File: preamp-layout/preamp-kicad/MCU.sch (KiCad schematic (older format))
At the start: 14 parts, among them J27 Conn_01x02_Female, J29 Conn_01x02_Female, J32 Conn_01x05_Female, J33 Conn_01x03_Male, J34 Conn_01x02_Male, J35 Conn_01x02_Male, U10 TCA9548APWR, U5 ESP32-DevKitC

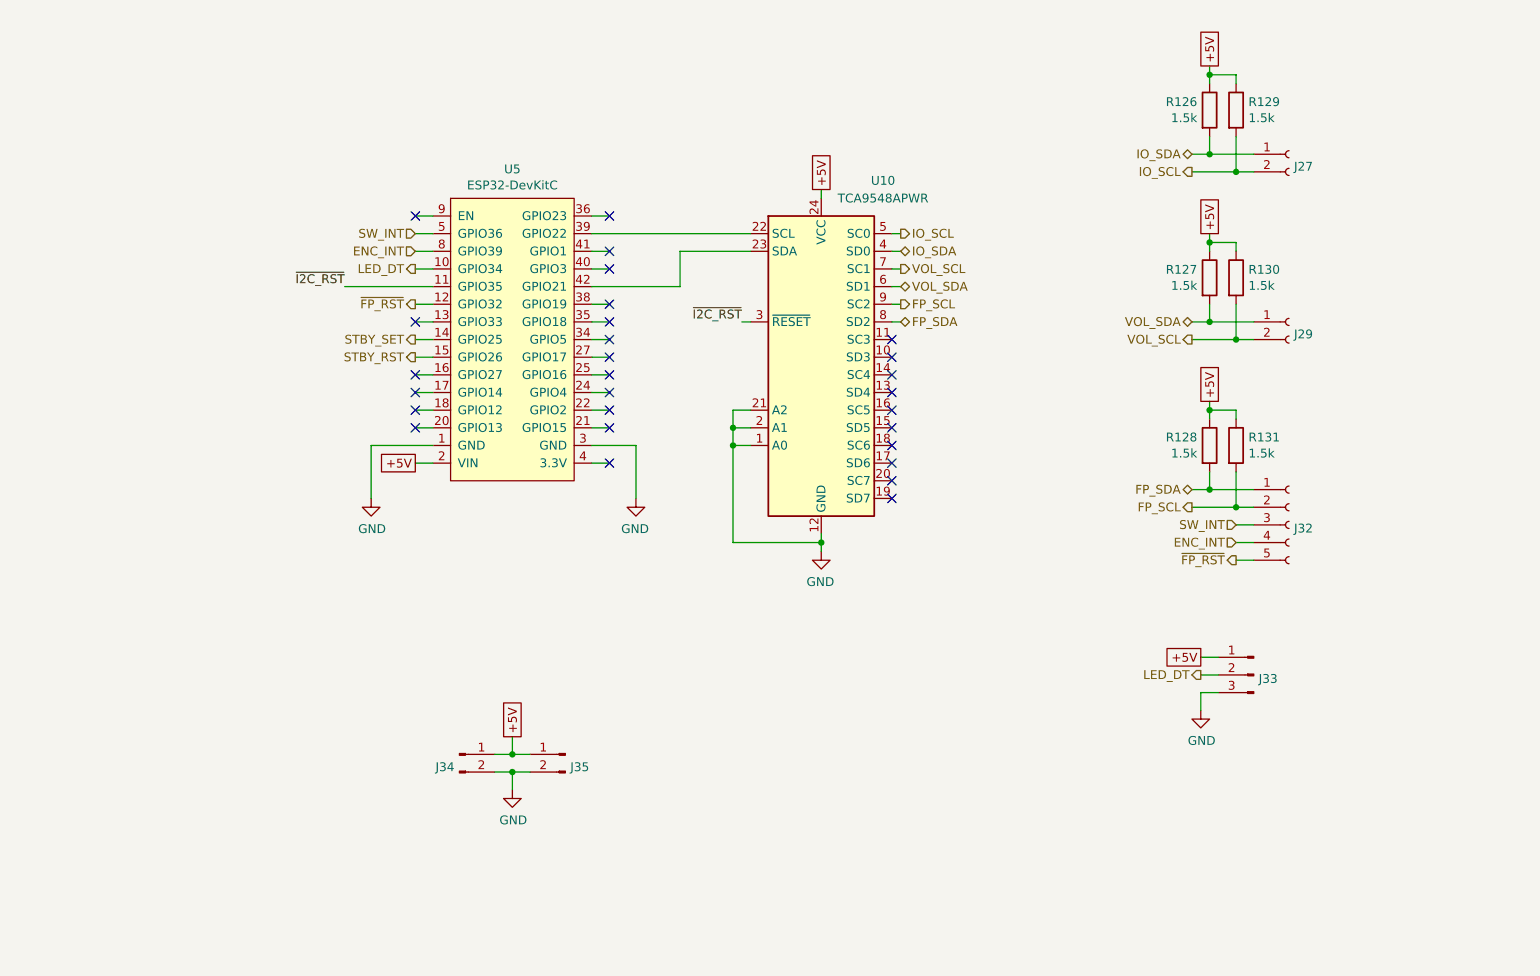
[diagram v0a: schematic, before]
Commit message: BOM Update
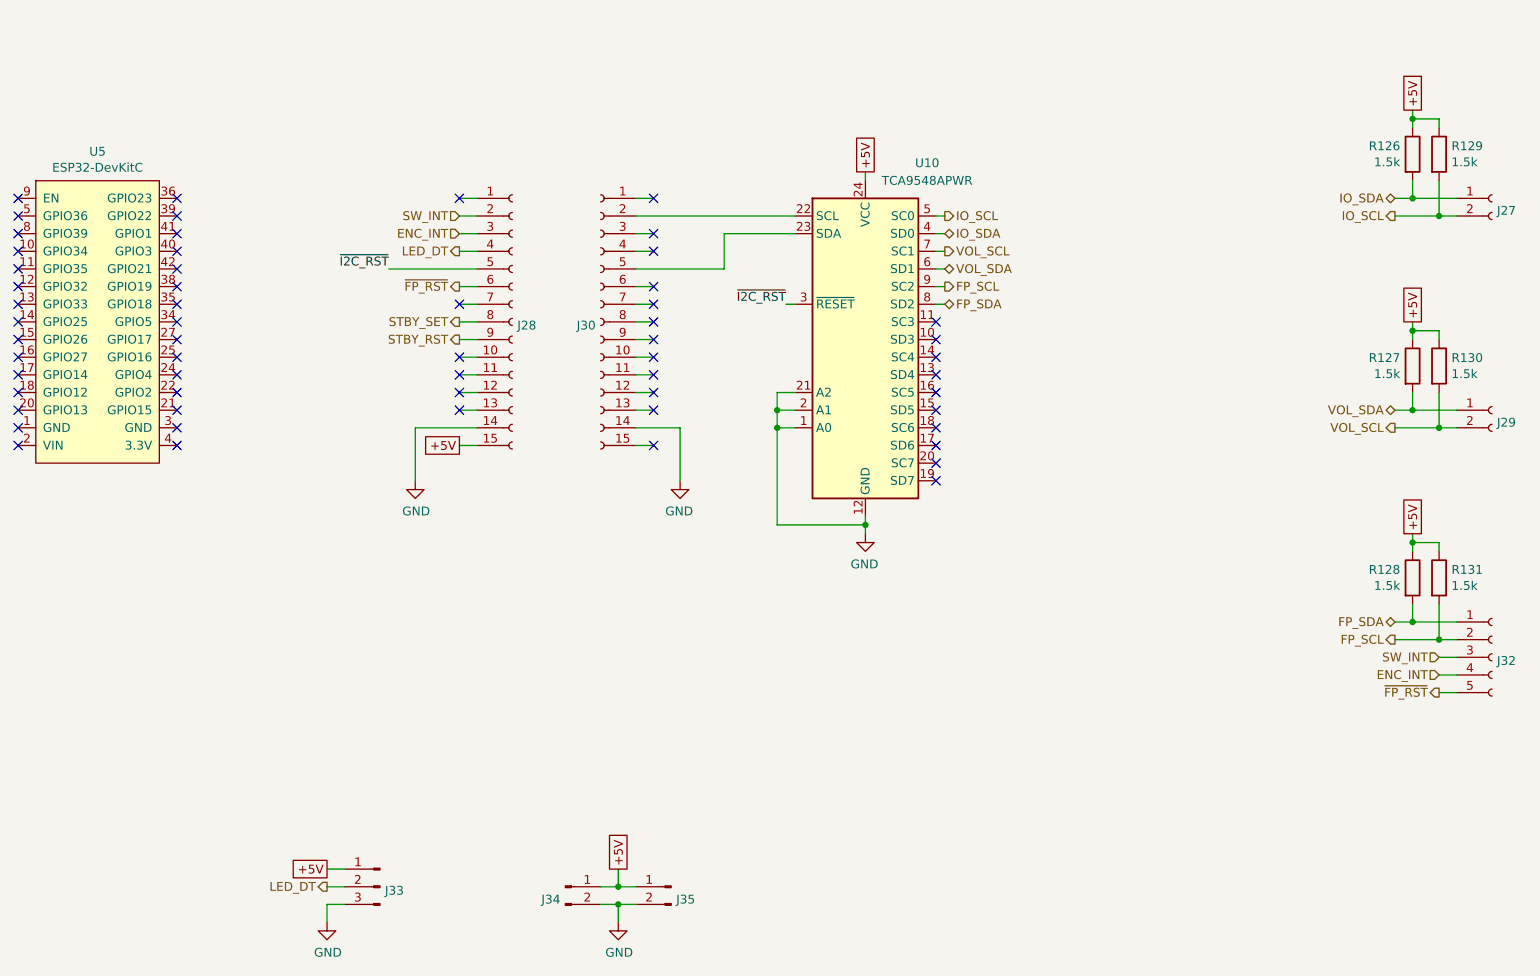
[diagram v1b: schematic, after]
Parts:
- added J28, J30: Conn_01x15_Female, symbol Connector:Conn_01x15_Female
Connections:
- net +5V: now also J28.15 (Pin_15); no longer U5.2 (VIN)
- net ENC_INT: now also J28.3 (Pin_3); no longer U5.8 (GPIO39)
- net GND: now also J28.14 (Pin_14), J30.14 (Pin_14); no longer U5.1 (GND), U5.3 (GND)
- net LED_DT: now also J28.4 (Pin_4); no longer U5.10 (GPIO34)
- net STBY_RST: now also J28.9 (Pin_9); no longer U5.15 (GPIO26)
- net STBY_SET: now also J28.8 (Pin_8); no longer U5.14 (GPIO25)
- net SW_INT: now also J28.2 (Pin_2); no longer U5.5 (GPIO36)
- net ~FP_RST: now also J28.6 (Pin_6); no longer U5.12 (GPIO32)
- net ~I2C_RST: now also J28.5 (Pin_5); no longer U5.11 (GPIO35)
- net at U10.22 (SCL): now also J30.2 (Pin_2); no longer U5.39 (GPIO22)
- net at U10.23 (SDA): now also J30.5 (Pin_5); no longer U5.42 (GPIO21)
- no-connect marks 28 -> 58
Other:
- moved on the sheet: J27, J29, J32, J33, J34, J35, R126, R127, R128, R129, R130, R131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
